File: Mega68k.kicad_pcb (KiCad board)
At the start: 2 copper layers, 101.9 x 53.6 mm, 27 parts, among them J1 CLK Select, J2 Ext CLK, J3 SPI, SW1 ARD RESET, U1 68000D, U2 AS6C4008-55PCN, U3 AS6C4008-55PCN, U4 74HC14, X1 CXO_DIP8

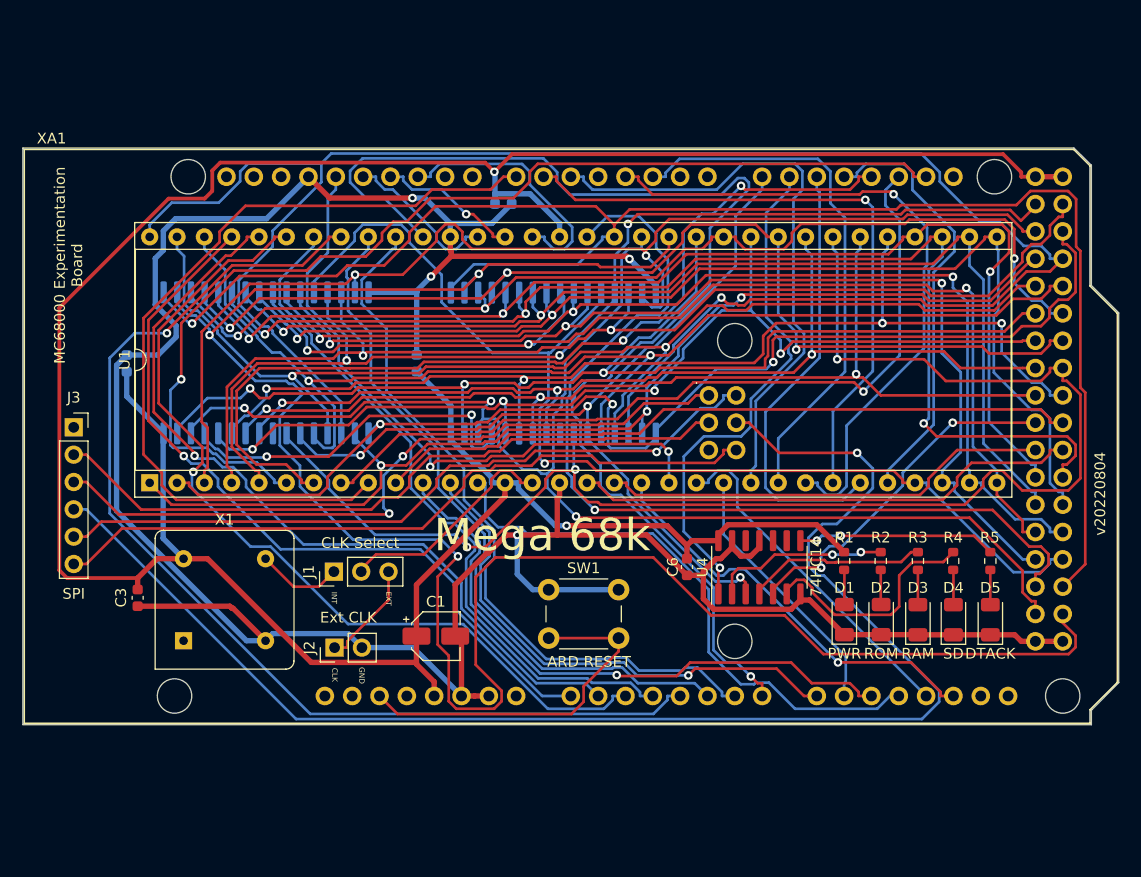
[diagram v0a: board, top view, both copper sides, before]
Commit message: Working freerun
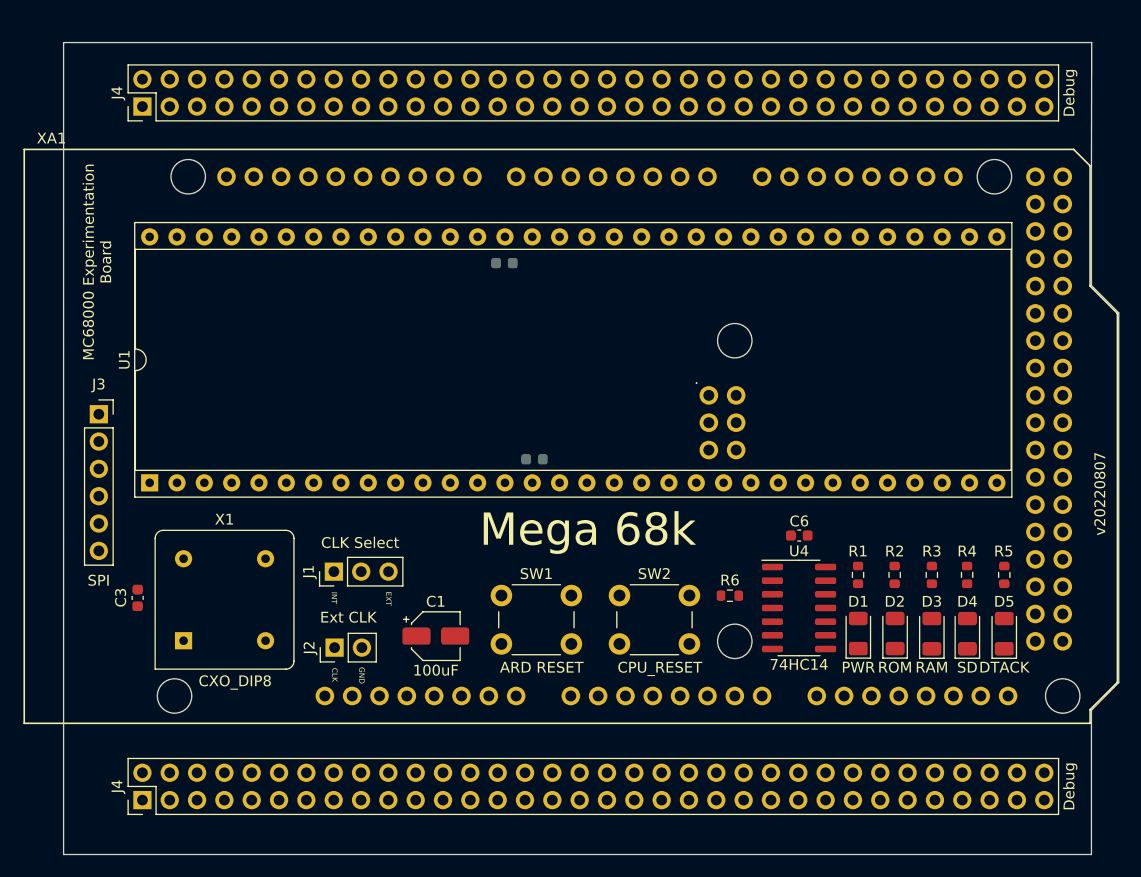
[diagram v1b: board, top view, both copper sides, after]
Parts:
- removed C4, C5: .1uF, Capacitor_SMD:C_0603_1608Metric
- removed U2, U3: AS6C4008-55PCN, Package_SO:SSOP-32_11.305x20.495mm_P1.27mm
- added C7: .1uF, Capacitor_SMD:C_0603_1608Metric, B.Cu at (95.6, 86.9)
- added J4: Debug, Connector_PinHeader_2.54mm:PinHeader_2x34_P2.54mm_Vertical, F.Cu at (59.2, 118.6)
- added J4: Debug, Connector_PinHeader_2.54mm:PinHeader_2x34_P2.54mm_Vertical, F.Cu at (59.2, 54.2)
- added R6: 10k, Resistor_SMD:R_0603_1608Metric, F.Cu at (113.8, 99.6)
- added SW2: CPU_RESET, Button_Switch_THT:SW_PUSH_6mm, F.Cu at (103.5, 99.6)
- moved C6 10.8 mm to (120.2, 94.0), turned to 180 degrees
- moved C2 5.51 mm to (92.8, 68.7)
- moved U4 5.28 mm to (120.2, 100.8), turned to 0 degrees
- moved SW1 4.43 mm to (92.6, 99.6)
- moved J3 2.64 mm to (55.1, 82.8)
- moved R2 1.83 mm to (129.1, 97.7)
- moved D1 1.83 mm to (125.7, 103.1)
- moved D2 1.83 mm to (129.1, 103.1)
- moved D3 1.83 mm to (132.6, 103.1)
- moved D4 1.83 mm to (135.9, 103.1)
- moved D5 1.83 mm to (139.3, 103.1)
- moved R1 1.83 mm to (125.7, 97.7)
- moved R3 1.83 mm to (132.6, 97.7)
- moved R4 1.83 mm to (135.8, 97.7)
- moved R5 1.83 mm to (139.3, 97.7)
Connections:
- XA1 pad D21: unconnected-(XA1-PadD21) -> /INT_CLK
- XA1 pad D4: unconnected-(XA1-PadD4) -> /CPU_RST
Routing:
- net VCC: track 273.0 -> 0.00 mm, vias 2 -> 0
- net GND: track 265.1 -> 0.00 mm, vias 4 -> 0
- net /A17: track 190.7 -> 0.00 mm, vias 3 -> 0
- net /D5: track 177.1 -> 0.00 mm, vias 1 -> 0
- net /A19: track 149.7 -> 0.00 mm, vias 1 -> 0
- net /A11: track 136.2 -> 0.00 mm, vias 3 -> 0
- net /SPI_MISO: track 134.0 -> 0.00 mm, vias 1 -> 0
- net /A18: track 122.7 -> 0.00 mm, vias 3 -> 0
- net /D15: track 115.2 -> 0.00 mm, vias 1 -> 0
- net /A7: track 111.8 -> 0.00 mm, vias 3 -> 0
- net /D7: track 110.9 -> 0.00 mm, vias 2 -> 0
- net /D2: track 110.6 -> 0.00 mm, vias 2 -> 0
- net /D6: track 109.6 -> 0.00 mm, vias 2 -> 0
- net /D3: track 109.3 -> 0.00 mm, vias 3 -> 0
- net /A16: track 108.8 -> 0.00 mm, vias 3 -> 0
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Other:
- board size 101.9 x 53.6 mm -> 98.1 x 75.5 mm
- board text added: "v20220807"
- board text removed: "v20220804"

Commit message: More tweaks to schematics before next rev V20220811
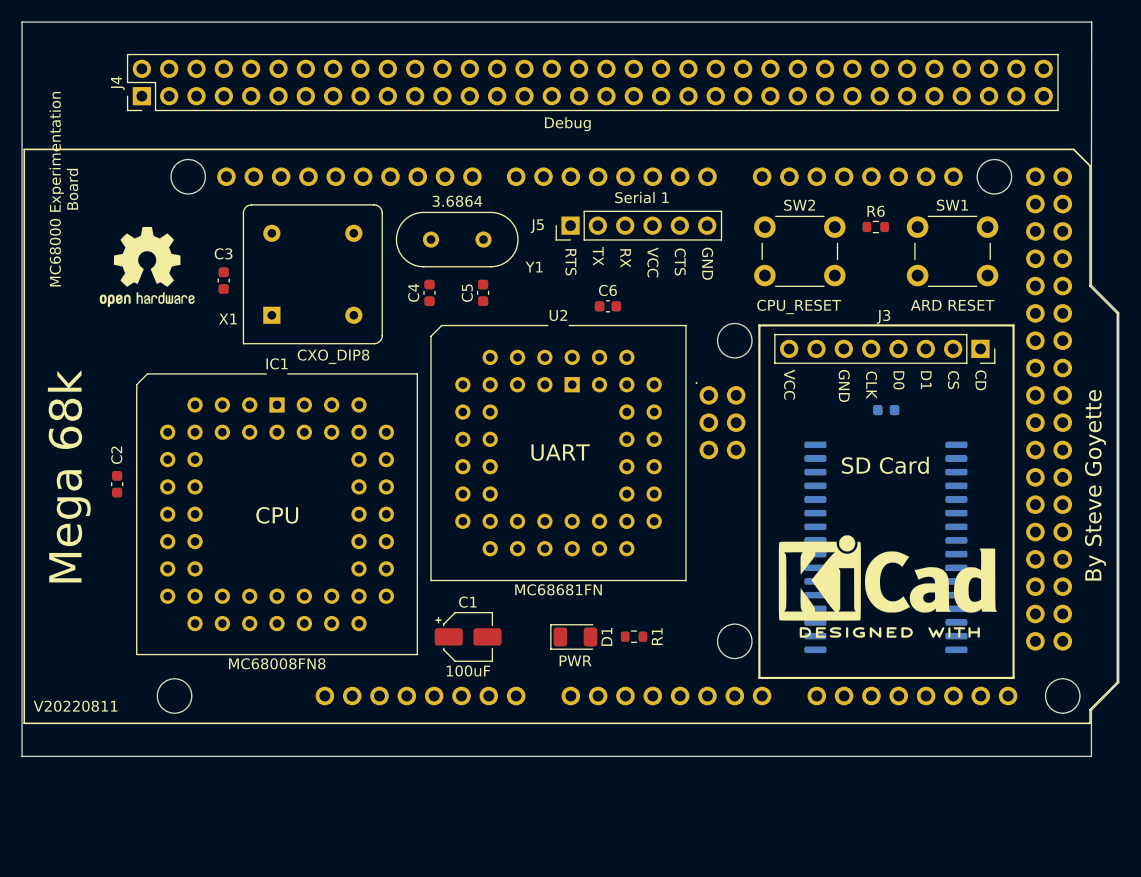
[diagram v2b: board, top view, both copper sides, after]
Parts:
- removed D2: ROM, LED_SMD:LED_1206_3216Metric
- removed D3: RAM, LED_SMD:LED_1206_3216Metric
- removed D4: SD, LED_SMD:LED_1206_3216Metric
- removed D5: DTACK, LED_SMD:LED_1206_3216Metric
- removed J1: CLK Select, Connector_PinHeader_2.54mm:PinHeader_1x03_P2.54mm_Vertical
- removed J2: Ext CLK, Connector_PinHeader_2.54mm:PinHeader_1x02_P2.54mm_Vertical
- removed the J4 at (59.2, 118.6)
- removed R2, R3, R4, R5: 220, Resistor_SMD:R_0603_1608Metric
- removed REF**: KiCad-Logo2_8mm_SilkScreen, Symbol:KiCad-Logo2_8mm_SilkScreen
- removed U4: 74HC14, Package_SO:SOIC-14_3.9x8.7mm_P1.27mm
- added C4: 12pf, Capacitor_SMD:C_0603_1608Metric, F.Cu at (85.9, 71.5)
- added C5: 12pf, Capacitor_SMD:C_0603_1608Metric, F.Cu at (90.9, 71.5)
- added IC1: MC68008FN8, Package_LCC:PLCC-52_THT-Socket, F.Cu at (71.7, 81.9)
- added J5: Serial 1, Connector_PinHeader_2.54mm:PinHeader_1x06_P2.54mm_Vertical, F.Cu at (99.0, 65.2)
- added Logo1: KiCad-Logo2_8mm_SilkScreen, Symbol:KiCad-Logo2_8mm_SilkScreen, F.Cu at (128.5, 97.9)
- added Logo2: OSHW-Logo2_9.8x8mm_SilkScreen, Symbol:OSHW-Logo2_9.8x8mm_SilkScreen, F.Cu at (59.6, 69.1)
- added U2: MC68681FN, Package_LCC:PLCC-44_THT-Socket, F.Cu at (99.1, 80.0)
- added Y1: 3.6864, Crystal:Crystal_HC49-U_Vertical, F.Cu at (90.9, 66.5)
- C2: moved to F.Cu
- J3: value SPI -> SD Card; footprint Connector_PinSocket_2.54mm:PinSocket_1x06_P2.54mm_Vertical -> Connector_PinSocket_2.54mm:PinSocket_1x08_P2.54mm_Vertical
- U1: value 68000D -> AS6C4008-55PCN; footprint Package_DIP:DIP-64_W22.86mm_Socket -> Package_SO:SSOP-32_11.305x20.495mm_P1.27mm; moved to B.Cu
- moved J3 82.2 mm to (137.1, 76.7), turned to -90 degrees
- moved U1 68.7 mm to (128.3, 95.1), turned to 180 degrees
- moved SW1 51.7 mm to (131.2, 65.4)
- moved C2 41.4 mm to (56.8, 89.3), turned to -90 degrees
- moved R6 36.9 mm to (127.4, 65.4)
- moved SW2 36.8 mm to (117.0, 65.4)
- moved C7 33.0 mm to (128.3, 82.4)
- moved X1 31.3 mm to (71.2, 73.6)
- moved C3 30.6 mm to (66.8, 70.3)
- moved C6 27.8 mm to (102.5, 72.7), turned to 0 degrees
- moved D1 26.3 mm to (99.4, 103.5), turned to 0 degrees
- moved R1 21.6 mm to (104.9, 103.4), turned to 180 degrees
- moved C1 3.00 mm to (89.5, 103.5)
- moved J4 0.97 mm to (59.1, 53.2)
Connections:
- C6 pad 2: GND -> unconnected-(C6-Pad2)
- J3 pad 1: /SDCARD_SEL -> unconnected-(J3-Pad1)
- J3 pad 2: /SPI_SCK -> /SDCS
- J3 pad 3: /SPI_MOSI -> /SDD1
- J3 pad 4: /SPI_MISO -> /SDD0
- J3 pad 5: /SPI_VCC -> /SDCLK
- J3 pad 6: /SPI_GND -> GND
- J4 pad 10: /A8 -> /A7
- J4 pad 11: /A9 -> /A8
- J4 pad 12: /A10 -> /A9
- J4 pad 13: /A11 -> /A10
- J4 pad 14: /A12 -> /A11
- J4 pad 15: /A13 -> /A12
- J4 pad 16: /A14 -> /A13
- J4 pad 17: /A15 -> /A14
- J4 pad 18: /A16 -> /A15
- J4 pad 19: /A17 -> /A16
- J4 pad 20: /A18 -> /A17
- J4 pad 21: /A19 -> /A18
- J4 pad 22: /A20 -> /A19
- J4 pad 23: /A21 -> /A20
- J4 pad 24: /A22 -> /A21
- J4 pad 25: /A23 -> unconnected-(J4-Pad25)
- J4 pad 26: /D0 -> unconnected-(J4-Pad26)
- J4 pad 27: /D1 -> /D0
- J4 pad 28: /D2 -> /D1
- J4 pad 29: /D3 -> /D2
- J4 pad 3: /A1 -> /A0
- J4 pad 30: /D4 -> /D3
- J4 pad 31: /D5 -> /D4
- J4 pad 32: /D6 -> /D5
- J4 pad 33: /D7 -> /D6
- J4 pad 34: /D8 -> /D7
- J4 pad 35: /D9 -> unconnected-(J4-Pad35)
- J4 pad 36: /D10 -> unconnected-(J4-Pad36)
- J4 pad 37: /D11 -> unconnected-(J4-Pad37)
- J4 pad 38: /D12 -> unconnected-(J4-Pad38)
- J4 pad 39: /D13 -> unconnected-(J4-Pad39)
- J4 pad 4: /A2 -> /A1
- J4 pad 40: /D14 -> unconnected-(J4-Pad40)
- J4 pad 41: /D15 -> unconnected-(J4-Pad41)
- J4 pad 45: /~{UDS} -> unconnected-(J4-Pad45)
- J4 pad 46: /~{LDS} -> /~{DS}
- J4 pad 47: /RESET -> /~{RESET}
- J4 pad 48: /HALT -> /~{HALT}
- J4 pad 49: /BERR -> /~{BERR}
- J4 pad 5: /A3 -> /A2
- J4 pad 50: /DTACK -> /~{DTACK}
- J4 pad 52: /VMA -> unconnected-(J4-Pad52)
- J4 pad 53: /BGACK -> /~{BGACK}
- J4 pad 54: /VPA -> /~{VPA}
- J4 pad 55: /BR -> /~{BR}
- J4 pad 56: /BG -> /~{BG}
- J4 pad 57: /IPL0 -> /~{IPL0}
- J4 pad 58: /IPL1 -> /~{IPL1}
- J4 pad 59: /IPL2 -> /~{IPL2}
- J4 pad 6: /A4 -> /A3
- J4 pad 65: /~{SDCARD_SEL} -> /~{RAM_WE}
- J4 pad 66: unconnected-(J4-Pad66) -> /~{OE}
- J4 pad 7: /A5 -> /A4
- J4 pad 8: /A6 -> /A5
- J4 pad 9: /A7 -> /A6
- U1 pad 1: /D4 -> /A18
- U1 pad 10: /DTACK -> /A2
- U1 pad 11: /BG -> /A1
- U1 pad 12: /BGACK -> /A0
- U1 pad 13: /BR -> /D0
- U1 pad 14: VCC -> /D1
- U1 pad 15: /CPU_CLK -> /D2
- U1 pad 17: /HALT -> /D3
- U1 pad 18: /RESET -> /D4
- U1 pad 19: /VMA -> /D5
- U1 pad 2: /D3 -> /A16
- U1 pad 20: /E -> /D6
- U1 pad 21: /VPA -> /D7
- U1 pad 22: /BERR -> /~{RAM_SEL}
- U1 pad 23: /IPL2 -> /A10
- U1 pad 24: /IPL1 -> /~{OE}
- U1 pad 25: /IPL0 -> /A11
- U1 pad 26: /FC2 -> /A9
- U1 pad 27: /FC1 -> /A8
- U1 pad 28: /FC0 -> /A13
- U1 pad 29: /A1 -> /~{RAM_WE}
- U1 pad 3: /D2 -> /A14
- U1 pad 30: /A2 -> /A17
- U1 pad 31: /A3 -> /A15
- U1 pad 32: /A4 -> VCC
- U1 pad 4: /D1 -> /A12
- U1 pad 5: /D0 -> /A7
- U1 pad 6: /AS -> /A6
- U1 pad 7: /UDS -> /A5
- U1 pad 8: /LDS -> /A4
- U1 pad 9: /R/W -> /A3
- X1 pad 5: /INT_CLK -> /CPU_CLK
- XA1 pad 5V2: /SPI_VCC -> unconnected-(XA1-Pad5V2)
- XA1 pad A0: /D8 -> /A16
- XA1 pad A1: /D9 -> /A17
- XA1 pad A10: /BG -> /~{BG}
- XA1 pad A11: /BR -> /~{BR}
- XA1 pad A12: /VPA -> /~{VPA}
- XA1 pad A13: /VMA -> /FC0
- XA1 pad A14: unconnected-(XA1-PadA14) -> /FC1
- XA1 pad A15: unconnected-(XA1-PadA15) -> /FC2
- XA1 pad A2: /D10 -> /A18
- XA1 pad A3: /D11 -> /A19
- XA1 pad A4: /D12 -> /A20
- XA1 pad A5: /D13 -> /A21
- XA1 pad A6: /D14 -> /E
- XA1 pad A7: /D15 -> unconnected-(XA1-PadA7)
- XA1 pad A8: /BGACK -> /~{BGACK}
- XA1 pad A9: /BERR -> /~{BERR}
- XA1 pad D10: /A21 -> /~{UART_SEL}
- XA1 pad D11: /A22 -> /~{RAM_SEL}
- XA1 pad D12: /A23 -> /~{DTACK_UART}
- XA1 pad D13: /E -> /~{RAM_WE}
- XA1 pad D14: /~{RAM_SEL} -> unconnected-(XA1-PadD14)
- XA1 pad D15: /~{ROM_SEL} -> unconnected-(XA1-PadD15)
- XA1 pad D16: /FC1 -> unconnected-(XA1-PadD16)
- XA1 pad D17: /FC0 -> unconnected-(XA1-PadD17)
- XA1 pad D18: /UDS -> unconnected-(XA1-PadD18)
- XA1 pad D19: /LDS -> unconnected-(XA1-PadD19)
- XA1 pad D2: /IPL1 -> /~{IPL1}
- XA1 pad D20: /AS -> unconnected-(XA1-PadD20)
- XA1 pad D21: /INT_CLK -> unconnected-(XA1-PadD21)
- XA1 pad D3: /IPL0 -> /~{IPL0}
- XA1 pad D30: /A16 -> /A15
- XA1 pad D31: /A15 -> /A14
- XA1 pad D32: /A14 -> /A13
- XA1 pad D33: /A13 -> /A12
- XA1 pad D34: /A12 -> /A11
- XA1 pad D35: /A11 -> /A10
- XA1 pad D36: /A10 -> /A9
- XA1 pad D37: /A9 -> /A8
- XA1 pad D38: /~{SDCARD_SEL} -> /~{OE}
- XA1 pad D39: /DTACK -> /~{DTACK}
- XA1 pad D40: /RESET -> /~{RESET}
- XA1 pad D41: /HALT -> /~{HALT}
- XA1 pad D42: /A8 -> /A7
- XA1 pad D43: /A7 -> /A6
- XA1 pad D44: /A6 -> /A5
- XA1 pad D45: /A5 -> /A4
- XA1 pad D46: /A4 -> /A3
- XA1 pad D47: /A3 -> /A2
- XA1 pad D48: /A2 -> /A1
- XA1 pad D49: /A1 -> /A0
- XA1 pad D5: /IPL2 -> /~{IPL2}
- XA1 pad D50: /A20 -> /SDD0
- XA1 pad D51: /A19 -> /SDD1
- XA1 pad D52: /A18 -> /SDCLK
- XA1 pad D53: /A17 -> /SDCS
- XA1 pad D6: /FC2 -> /~{AS}
- XA1 pad D7: /R/W -> /~{DS}
- XA1 pad D8: unconnected-(XA1-PadD8) -> /R~{W}
- XA1 pad D9: unconnected-(XA1-PadD9) -> /CPU_CLK
- XA1 pad GND4: /SPI_GND -> unconnected-(XA1-PadGND4)
- XA1 pad MISO: /SPI_MOSI -> unconnected-(XA1-PadMISO)
- XA1 pad MOSI: /SPI_MISO -> unconnected-(XA1-PadMOSI)
- XA1 pad SCK: /SPI_SCK -> unconnected-(XA1-PadSCK)
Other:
- board size 98.1 x 75.5 mm -> 101.9 x 68.2 mm
- board text added: "CD"
- board text added: "CPU"
- board text added: "CS"
- board text added: "CTS"
- board text added: "D0"
- board text added: "D1"
- board text added: "RTS"
- board text added: "RX"
- board text added: "SD Card"
- board text added: "TX"
- board text added: "UART"
- board text added: "V20220811"
- board text added: "VCC"
- board text removed: "EXT"
- board text removed: "INT"
- board text removed: "v20220807"
